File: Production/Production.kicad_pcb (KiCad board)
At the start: 2 copper layers, 37 x 35 mm, 36 parts, among them IC1 MAX3323EEPE+, J1 530480510, J13 FH34SRJ-16S-0.5SH_50_, J2 530480410, J3 USB4085-GF-A_REVB, J6 Program, U1 BD33FC0FP-E2, U2 ADR02AUJZ-REEL7, U3 ATSAMD21G18A-AUT, Y1 32.768, 12.5pF

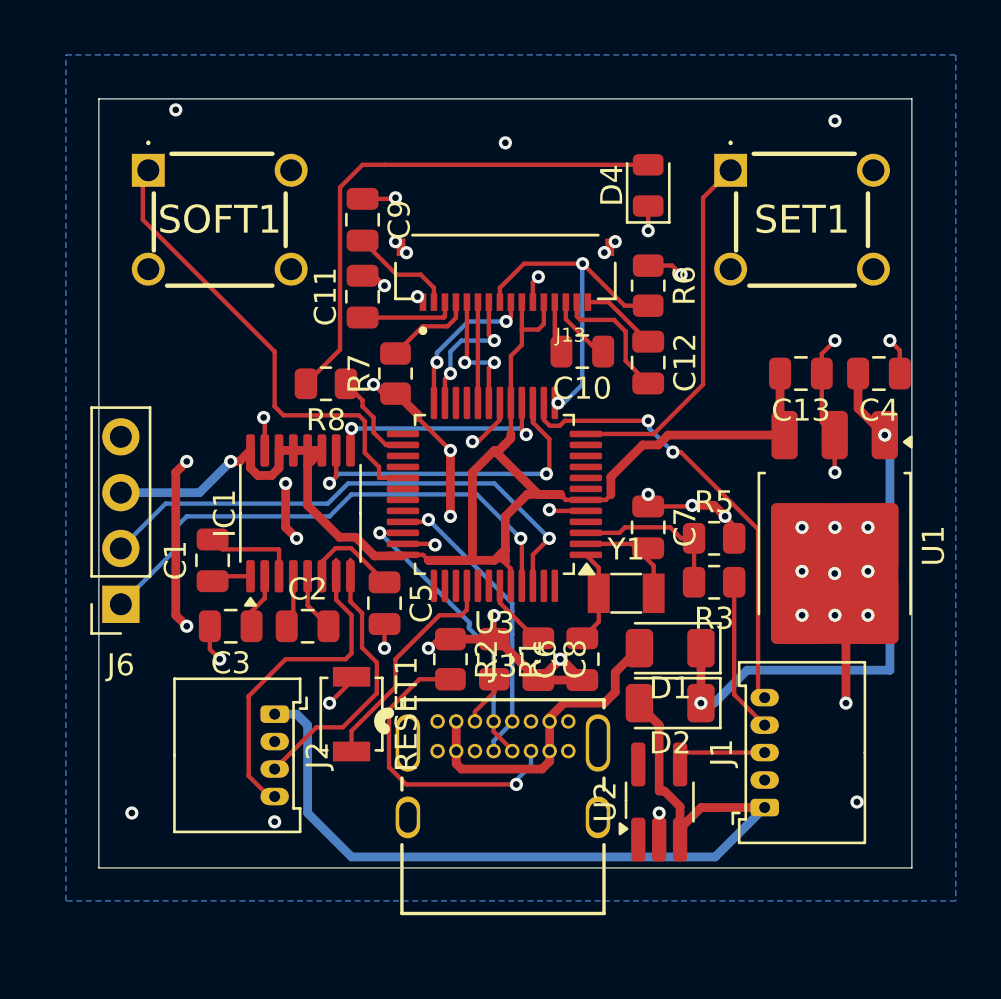
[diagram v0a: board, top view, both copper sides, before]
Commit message: I layout
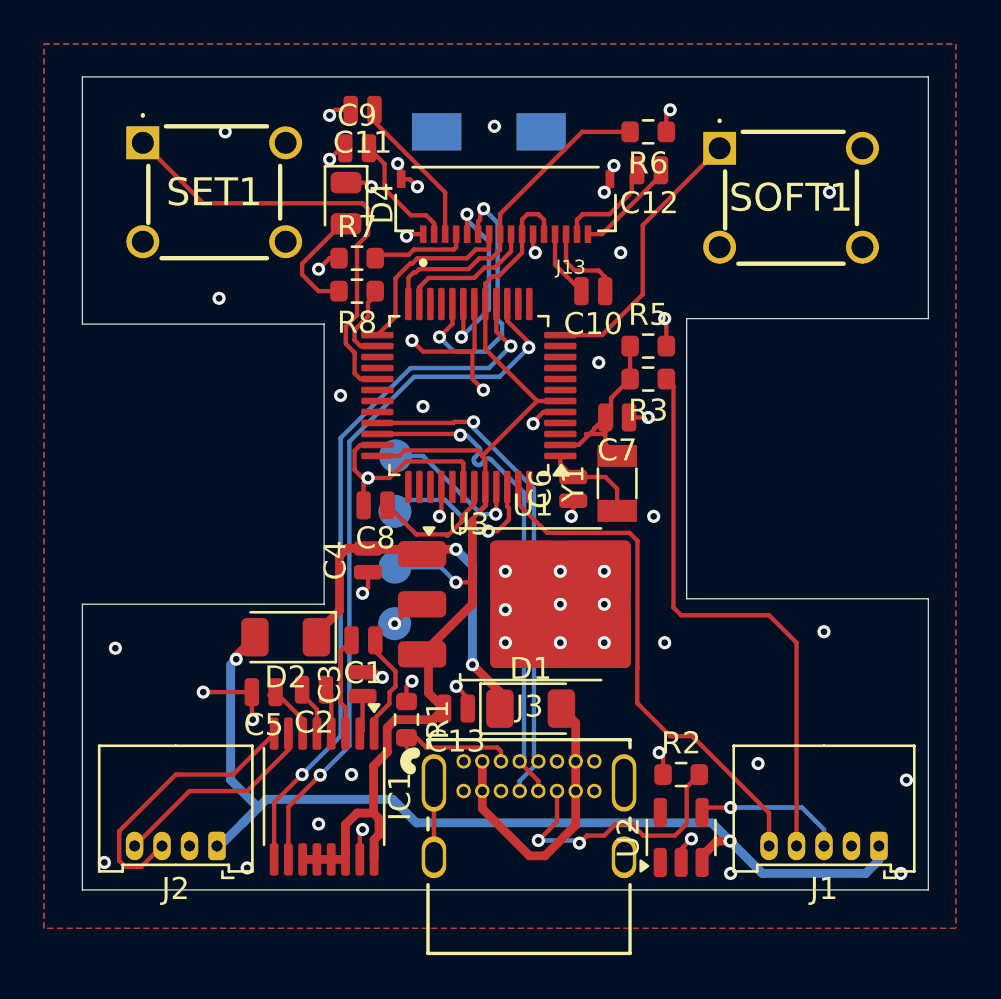
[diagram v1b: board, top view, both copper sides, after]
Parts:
- removed J6: Program, Connector_PinSocket_2.54mm:PinSocket_1x04_P2.54mm_Vertical
- added REF**: TestPoint_Pad_D1.5mm, TestPoint:TestPoint_Pad_D1.5mm, B.Cu at (101.5, 84.3)
- added REF**: TestPoint_Pad_D1.5mm, TestPoint:TestPoint_Pad_D1.5mm, B.Cu at (101.5, 89.4)
- added REF**: TestPoint_Pad_D1.5mm, TestPoint:TestPoint_Pad_D1.5mm, B.Cu at (101.5, 86.8)
- added REF**: TestPoint_Pad_D1.5mm, TestPoint:TestPoint_Pad_D1.5mm, B.Cu at (101.5, 81.8)
- C1, C10, C11, C12, C13, C2, C3, C4, C5, C6, C7, C8, C9: footprint Capacitor_SMD:C_0805_2012Metric -> Capacitor_SMD:C_0504_1310Metric
- J2: footprint Connector_Molex:Molex_PicoBlade_53048-0410_1x04_P1.25mm_Horizontal -> Connector_Molex_2:Molex_PicoBlade_53048-0410_1x04_P1.25mm_Horizontal
- R1, R2, R3, R5, R6, R7, R8: footprint Resistor_SMD:R_0805_2012Metric -> Resistor_SMD:R_0603_1608Metric
- RESET1: footprint Button_Switch_SMD:SW_SPST_B3U-1000P -> Button_Switch_SMD:SW_SPST_B3U-3000P; moved to B.Cu
- U2: footprint Package_TO_SOT_SMD:TSOT-23-5_HandSoldering -> Package_TO_SOT_SMD:TSOT-23-5
- moved RESET1 27.2 mm to (105.8, 67.0), turned to 180 degrees
- moved SET1 26.8 mm to (90.0, 67.5)
- moved SOFT1 26.0 mm to (116.2, 67.8)
- moved C4 24.8 mm to (100.2, 86.5), turned to 90 degrees
- moved C13 21.9 mm to (104.2, 93.2)
- moved D2 17.8 mm to (96.5, 90.0)
- moved U1 14.0 mm to (107.8, 88.5), turned to 0 degrees
- moved D4 13.8 mm to (99.2, 70.2), turned to -90 degrees
- moved IC1 12.9 mm to (98.2, 97.2), turned to -90 degrees
- moved R2 11.7 mm to (114.5, 96.2), turned to 0 degrees
- moved C8 10.2 mm to (100.6, 84.0), turned to 180 degrees
- moved R3 9.72 mm to (113.0, 78.2)
- moved R5 9.25 mm to (113.0, 76.8)
- moved C12 8.75 mm to (113.0, 68.8), turned to 180 degrees
- moved C11 8.50 mm to (100.0, 66.0), turned to 180 degrees
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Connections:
- R8 pad 1: TXLED -> SETLED
- U3 pad 12: SETBTN -> SOFTBTN
- U3 pad 13: OLED_RST -> unconnected-(U3-PA08-Pad13)
- U3 pad 14: RUN -> unconnected-(U3-PA09-Pad14)
- U3 pad 23: OLED_DC -> OLED_CS
- U3 pad 24: OLED_CS -> OLED_RST
- U3 pad 25: RS_INVALID -> OLED_DC
- U3 pad 29: SOFTBTN -> SETBTN
- U3 pad 47: unconnected-(U3-PB02-Pad47) -> RUN
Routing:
- net GND: track 72.4 -> 48.2 mm, vias 50 -> 57
- net ROUT1: track 10.3 -> 32.1 mm
- net ZOOM: track 7.07 -> 26.0 mm
- net Net-(D4-A): track 23.5 -> 5.24 mm
- net SWCLK: track 23.9 -> 6.91 mm
- net SWDIO: track 24.2 -> 7.79 mm
- net TIN1: track 16.8 -> 32.5 mm
- net +3V3: track 67.2 -> 53.9 mm
- net SOFTBTN: track 21.8 -> 12.6 mm
- net D-: track 13.7 -> 22.8 mm
- net D+: track 13.7 -> 22.7 mm
- net RST: track 10.3 -> 1.37 mm, vias 0 -> 1
- net VIN: track 25.8 -> 17.9 mm
- net SCK: track 4.59 -> 12.5 mm, vias 0 -> 2
- net TOUT1: track 15.2 -> 9.55 mm
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- added copper zone on F.Cu, net GND
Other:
- board size 37 x 35 mm -> 38.5 x 37 mm
